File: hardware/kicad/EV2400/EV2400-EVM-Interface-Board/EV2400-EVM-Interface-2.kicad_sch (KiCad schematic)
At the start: 75 parts, among them J2 Conn_01x04, J3 Conn_01x04, J4 Conn_01x04, J5 Conn_01x04, Q1 BSS209PW, Q2 BSS209PW, Q3 BSS209PW, Q4 BSS209PW, Q5 BSS209PW, Q6 BSS209PW, Q7 2N7002W, Q8 2N7002W, Q9 2N7002W, U3 TPS76333DBV, U4 ST2329BQTR, U5 ST2329BQTR, U6 ST2329BQTR, U7 TPS79650DCQ, U8 TPS2113APWR

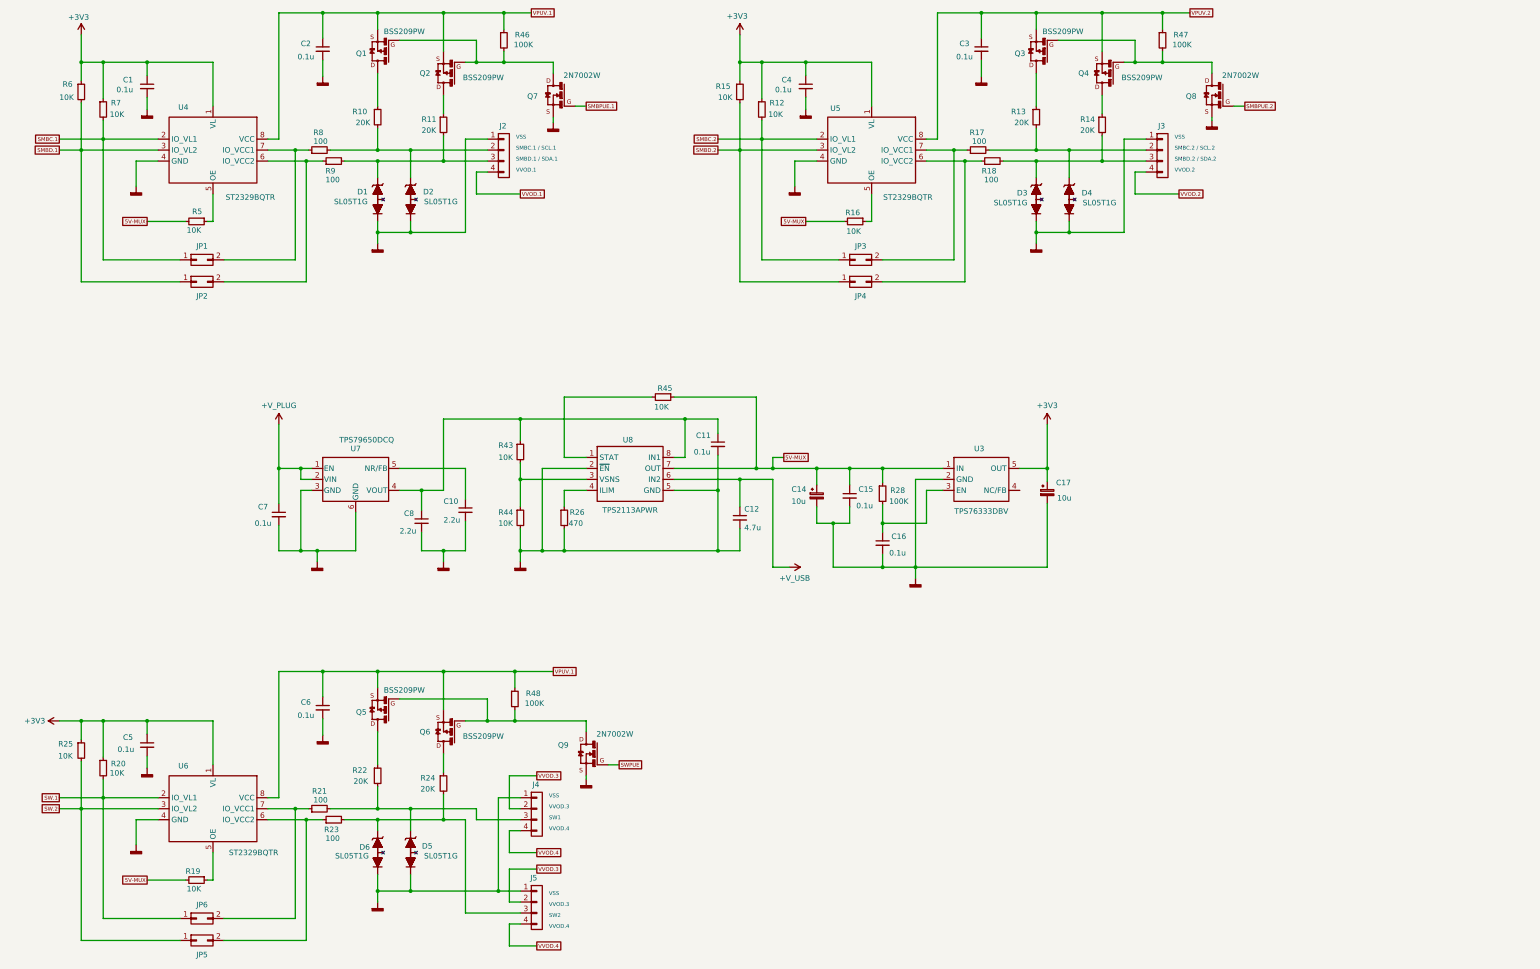
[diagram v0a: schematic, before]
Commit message: Update EV2400 kicad files
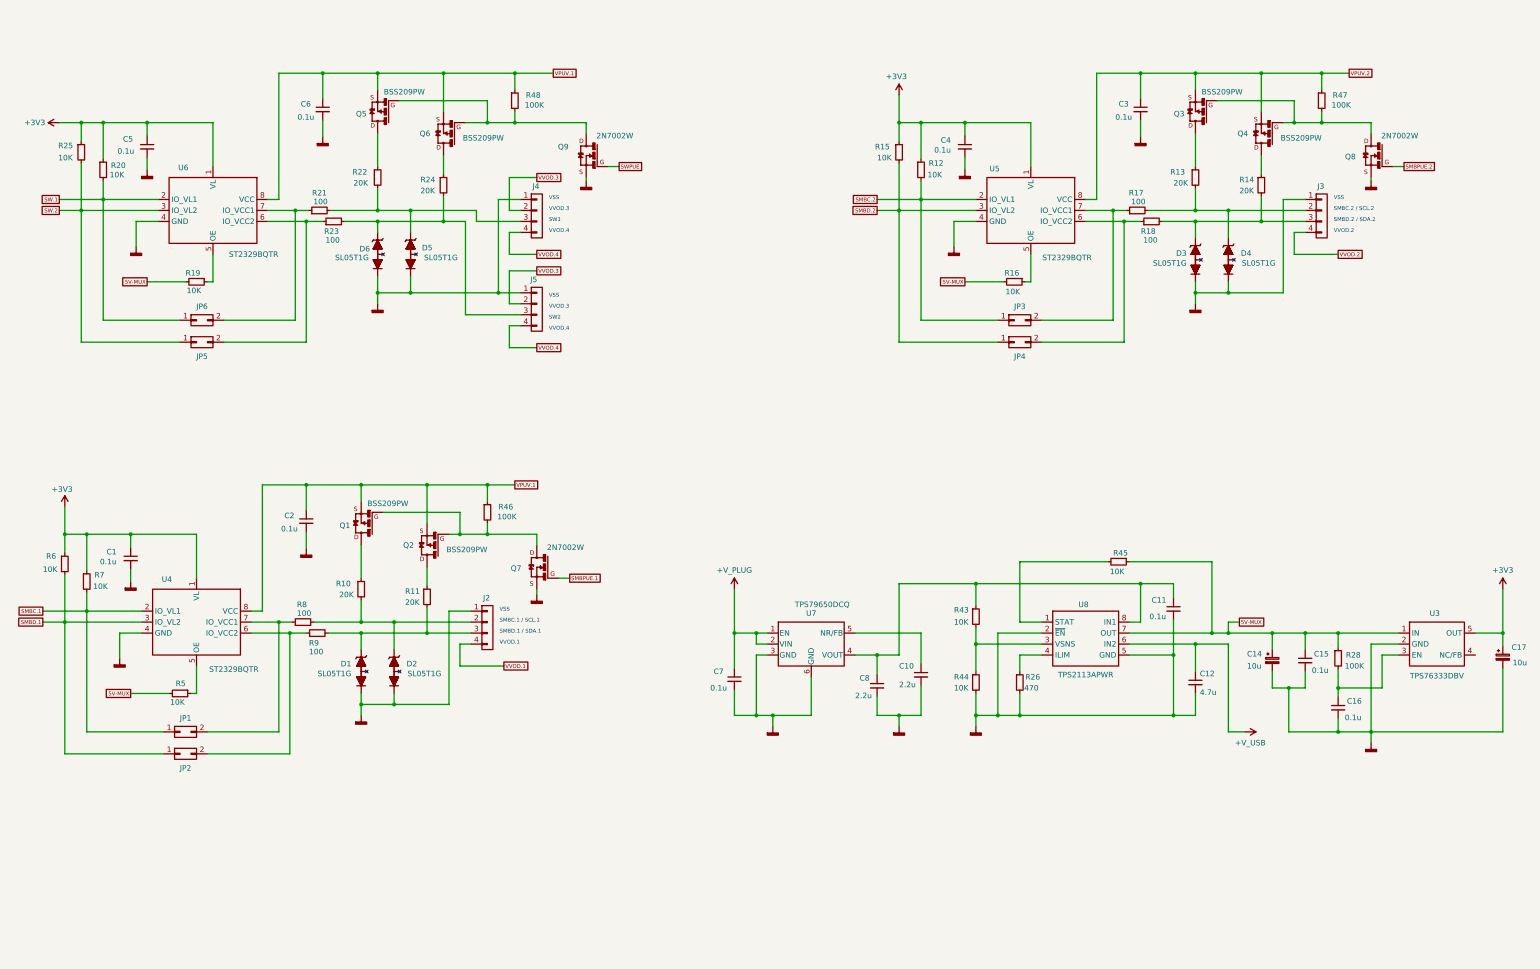
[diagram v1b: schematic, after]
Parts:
- C1, C10, C11, C12, C15, C16, C2, C3, C4, C5, C6, C7, C8: symbol EV2400-EVM-Interface-Board-rescue:C_Small-EV2400-Components -> EV2400-Components:C_Small
- C14, C17: symbol EV2400-EVM-Interface-Board-rescue:CP_Small-EV2400-Components -> EV2400-Components:CP_Small
- D1, D2, D3, D4, D5, D6: symbol EV2400-EVM-Interface-Board-rescue:SL05T1G-EV2400-Components -> EV2400-Components:SL05T1G; Description_1 (none) -> 300 Watt, SOT-23 Low Capacitance TVS for High Speed Line Pr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
- J2, J3, J4, J5: symbol EV2400-EVM-Interface-Board-rescue:Conn_01x04-EV2400-Components -> EV2400-Components:Conn_01x04
- JP1, JP2, JP5, JP6: symbol EV2400-EVM-Interface-Board-rescue:Conn_02x01-EV2400-Components -> EV2400-Components:Conn_02x01
- Q1, Q2, Q5, Q6: symbol EV2400-EVM-Interface-Board-rescue:P-CHANNEL-MOSFET-EV2400-Components -> EV2400-Components:P-CHANNEL-MOSFET
- Q7, Q8, Q9: symbol EV2400-EVM-Interface-Board-rescue:N-CHANNEL-MOSFET-EV2400-Components -> EV2400-Components:N-CHANNEL-MOSFET
- R10, R11, R12, R13, R14, R15, R16, R17, R18, R19, R20, R21, R22, R23, R24, R25, R26, R28, R43, R44, R45, R46, R47, R48, R5, R6, R7, R8, R9: symbol EV2400-EVM-Interface-Board-rescue:R_Small-EV2400-Components -> EV2400-Components:R_Small
- U3: symbol EV2400-EVM-Interface-Board-rescue:TPS76333DBV-EV2400-Components -> EV2400-Components:TPS76333DBV; Description_1 (none) -> Low Iq, 150-mA, Low-Dropout Linear Regulators
- U4, U5, U6: symbol EV2400-EVM-Interface-Board-rescue:ST2329BQTR-EV2400-Components -> EV2400-Components:ST2329BQTR; Description_1 (none) -> Translation - Voltage Levels 2-Bit Dual LVL Trans 18Mbps 5.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
- U7: symbol EV2400-EVM-Interface-Board-rescue:TPS79650DCQ-EV2400-Components -> EV2400-Components:TPS79650DCQ; Description_1 (none) -> Ultralow-Noise, High PSRR, Fast, RF, 1-A Low-Dropout Linear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
- U8: symbol EV2400-EVM-Interface-Board-rescue:TPS2113APWR-EV2400-Components -> EV2400-Components:TPS2113APWR; Description_1 (none) -> AUTOSWITCHING POWER MUX
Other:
- moved on the sheet: C1, C10, C11, C12, C14, C15, C16, C17, C2, C3, C4, C5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
